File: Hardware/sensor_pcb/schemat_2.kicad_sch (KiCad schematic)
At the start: 40 parts, among them J7 SENSOR_CONN, J8 ToF Sensor

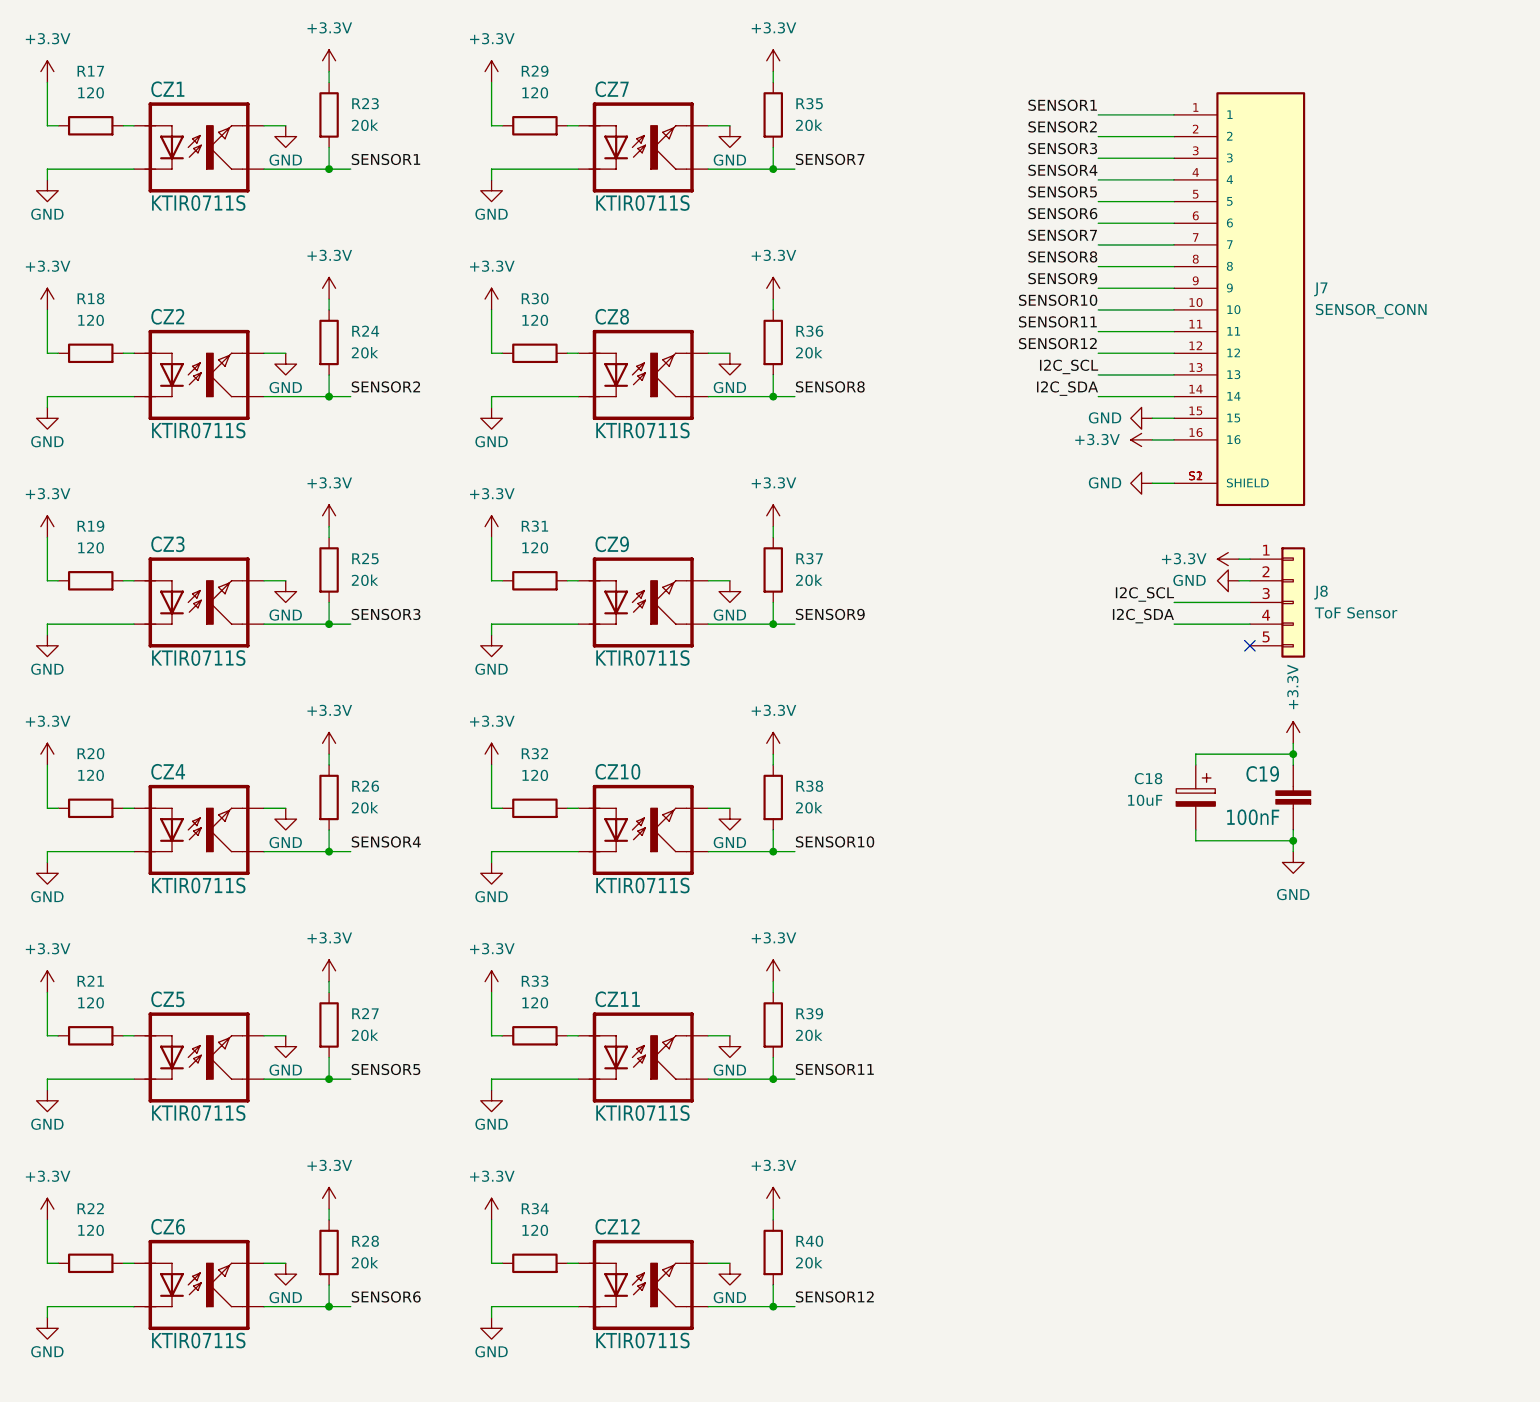
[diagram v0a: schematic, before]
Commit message: Minor fixes in schematics, added gerbers and schematics pdfs
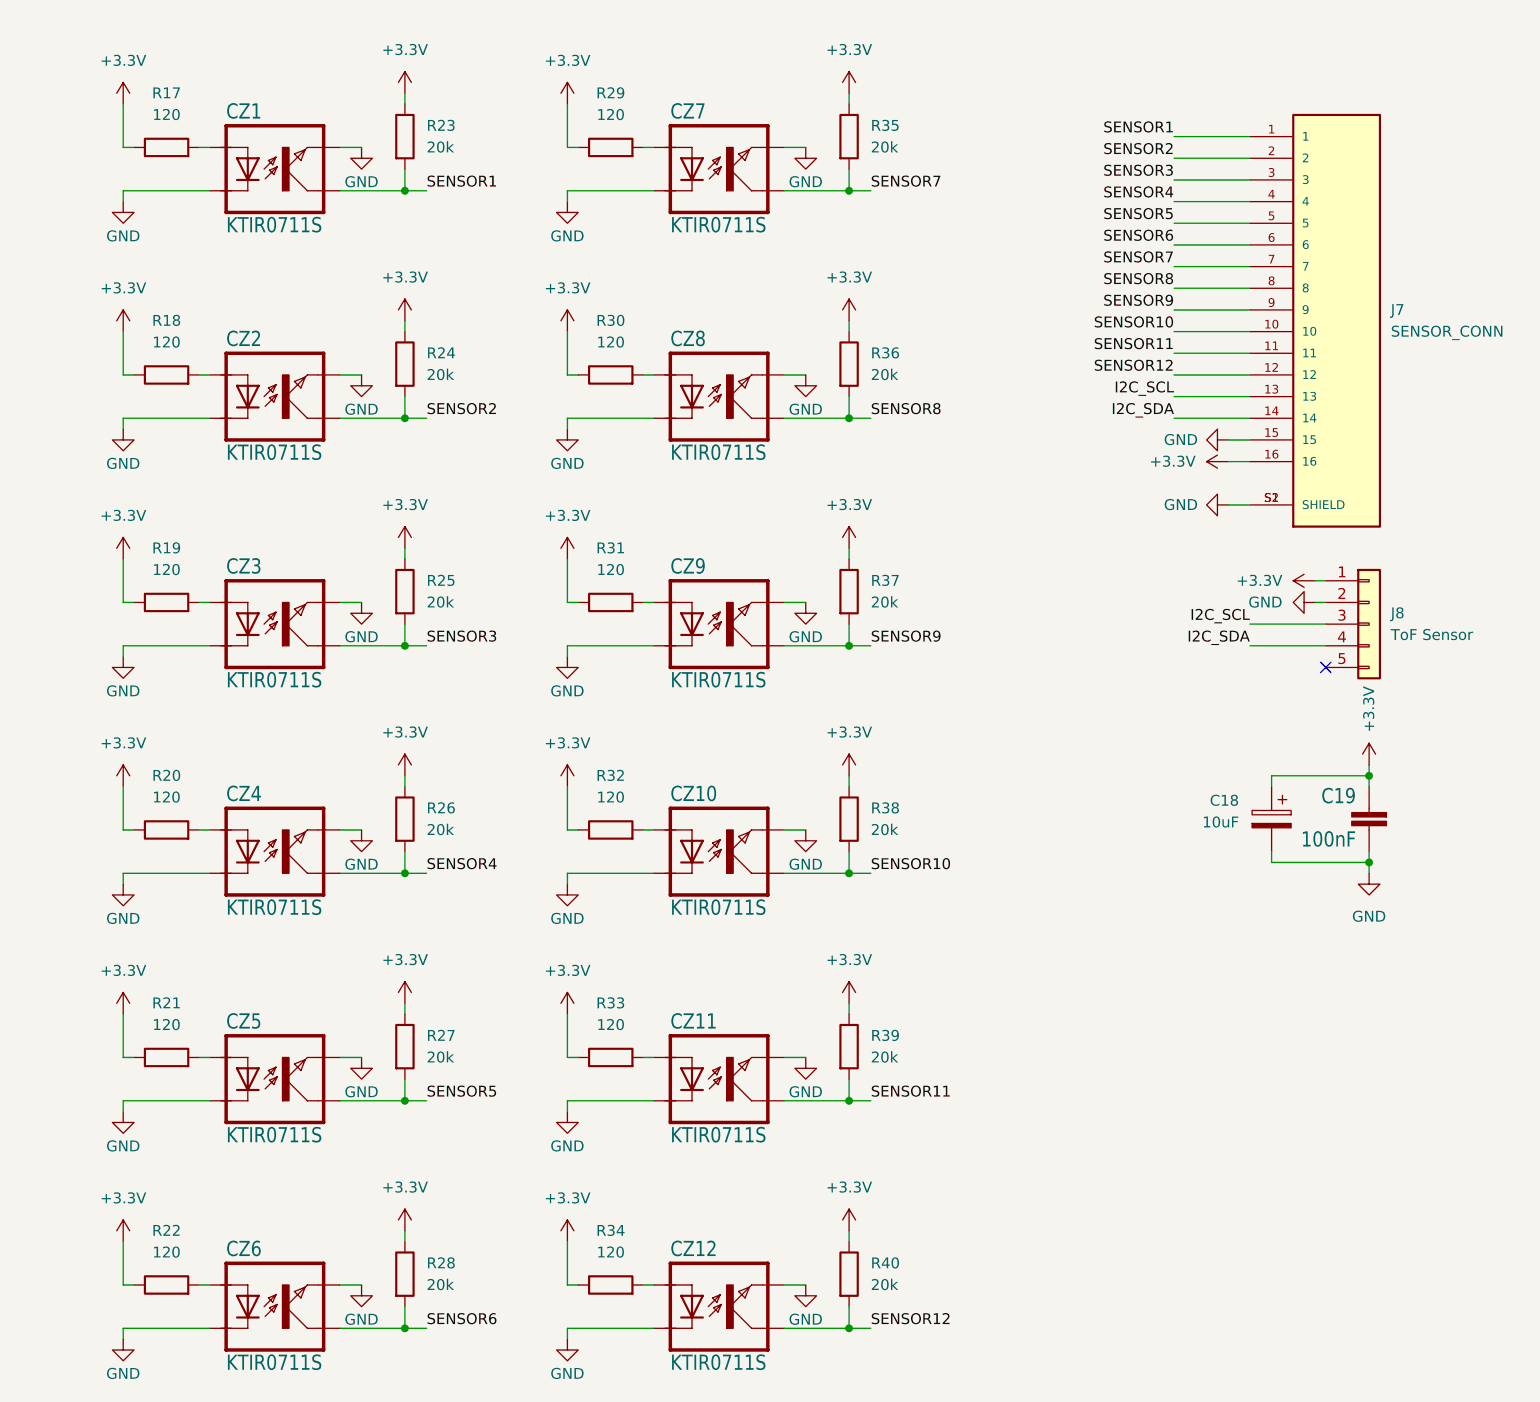
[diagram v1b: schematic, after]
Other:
- moved on the sheet: C18, C19, CZ1, CZ10, CZ11, CZ12, CZ2, CZ3, CZ4, CZ5, CZ6, CZ7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
